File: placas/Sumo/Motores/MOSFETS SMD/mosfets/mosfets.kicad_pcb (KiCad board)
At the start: 2 copper layers, 37.3 x 39.4 mm, 18 parts, among them J1 Screw_Terminal_01x02, J3 Screw_Terminal_01x02, J5 Conn_01x06_Pin, Q1 IRLZ44N, Q2 IRLZ44N, Q3 IRLZ44N, Q4 IRLZ44N, U1 HIP4082xP

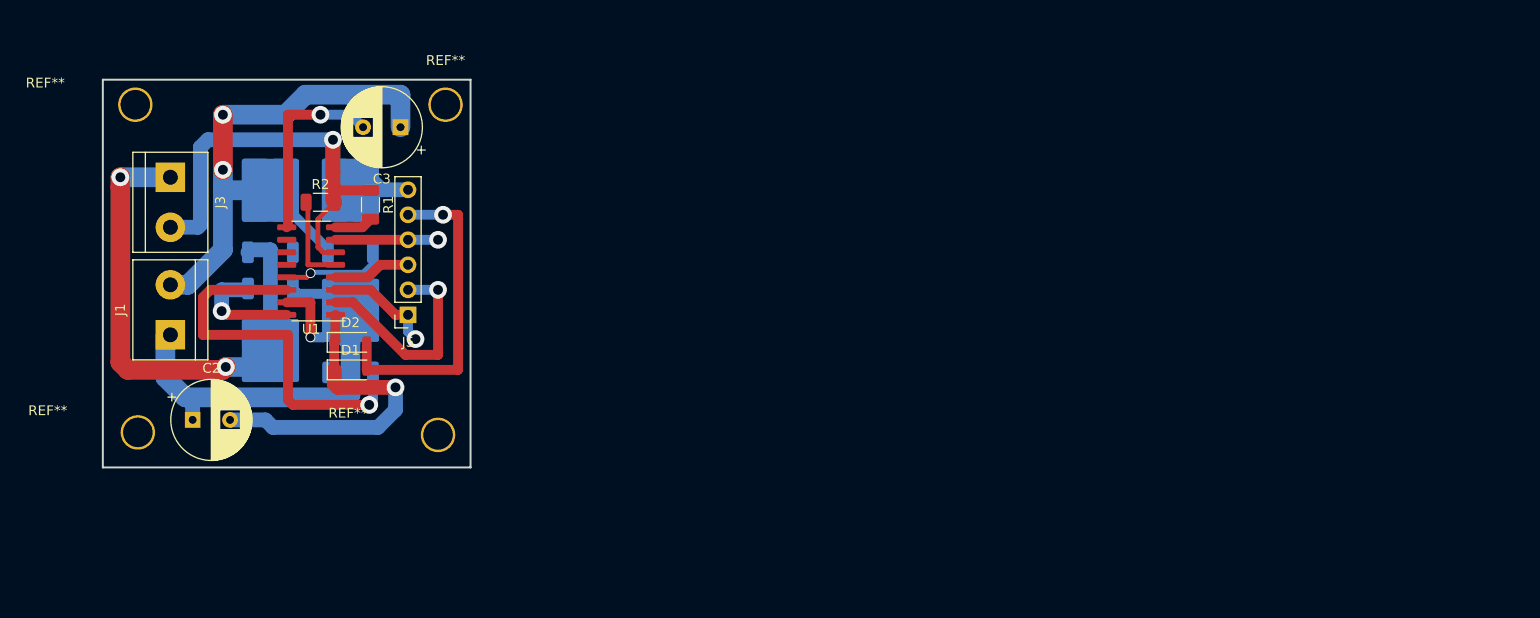
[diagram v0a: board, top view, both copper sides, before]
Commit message: dfg
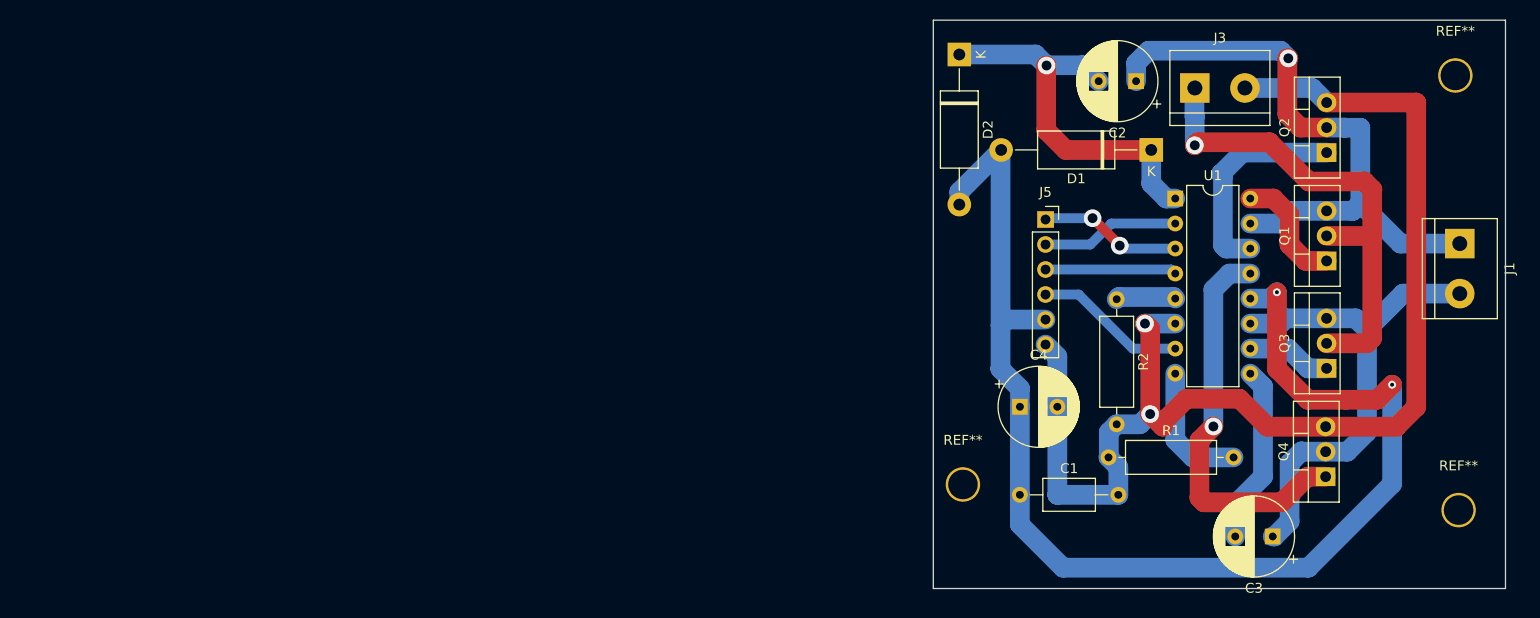
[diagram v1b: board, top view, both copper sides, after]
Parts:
- removed the REF** at (54.6, 52.8)
- removed the REF** at (24.1, 52.6)
- removed the REF** at (23.9, 19.3)
- removed the REF** at (55.4, 19.3)
- added C1: C, Capacitor_THT:C_Axial_L5.1mm_D3.1mm_P10.00mm_Horizontal, F.Cu at (113.7, 58.9)
- added C4: 47nf, Capacitor_THT:CP_Radial_D8.0mm_P3.80mm, F.Cu at (113.7, 50.0)
- added REF**: MountingHole_3.5mm_Pad, MountingHole:MountingHole_3.5mm_Pad, F.Cu at (158.2, 60.4)
- added REF**: MountingHole_3.5mm_Pad, MountingHole:MountingHole_3.5mm_Pad, F.Cu at (157.9, 16.3)
- added REF**: MountingHole_3.5mm_Pad, MountingHole:MountingHole_3.5mm_Pad, F.Cu at (107.9, 57.8)
- C2, C3: value C_Polarized -> 47nf
- D1, D2: footprint Diode_SMD:D_SOD-123 -> Diode_THT:D_DO-15_P15.24mm_Horizontal
- Q1, Q2, Q3, Q4: footprint Package_TO_SOT_SMD:TO-252-2 -> Package_TO_SOT_THT:TO-220-3_Vertical; moved to F.Cu
- R1, R2: value R -> 36k; footprint Resistor_SMD:R_1206_3216Metric -> Resistor_THT:R_Axial_DIN0309_L9.0mm_D3.2mm_P12.70mm_Horizontal
- U1: footprint Package_SO:SOIC-16_3.9x9.9mm_P1.27mm -> Package_DIP:DIP-16_W7.62mm
- moved J1 131.3 mm to (158.4, 33.4), turned to -90 degrees
- moved Q3 108.6 mm to (144.8, 46.0)
- moved Q1 107.5 mm to (144.8, 35.1), turned to 90 degrees
- moved J3 104.4 mm to (131.5, 17.6), turned to 0 degrees
- moved Q4 102.9 mm to (144.7, 57.0)
- moved C2 101.8 mm to (125.5, 16.9), turned to 180 degrees
- moved Q2 100.6 mm to (144.8, 24.1)
- moved C3 97.8 mm to (139.4, 63.1)
- moved U1 88.1 mm to (129.5, 28.8), turned to 0 degrees
- moved D1 84.3 mm to (127.0, 23.9), turned to 180 degrees
- moved R2 81.4 mm to (123.5, 39.0), turned to -90 degrees
- moved R1 79.2 mm to (122.7, 55.1), turned to 0 degrees
- moved D2 68.4 mm to (107.5, 14.2), turned to -90 degrees
- moved J5 65.5 mm to (116.3, 30.9), turned to 0 degrees
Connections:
- Q3 pad 2: Net-(J1-Pin_2) -> VDD
- Q3 pad 3: VDD -> Net-(J1-Pin_2)
- Q4 pad 2: GND -> Net-(J1-Pin_2)
- Q4 pad 3: Net-(J1-Pin_2) -> GND
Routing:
- net +5V: track 32.9 -> 128.6 mm, vias 1 -> 2
- net GND: track 53.7 -> 126.1 mm, vias 1 -> 2
- net Net-(Q4-G): track 10.4 -> 40.2 mm
- net Net-(Q2-G): track 39.8 -> 21.9 mm, vias 1 -> 0
- net Net-(U1-DIS): track 3.90 -> 13.4 mm
- net Net-(Q3-G): track 0.00 -> 8.58 mm
- net Net-(J5-Pin_2): track 22.3 -> 14.1 mm, vias 1 -> 0
- net Net-(D1-K): track 33.6 -> 39.9 mm
- net Net-(J1-Pin_1): track 69.0 -> 63.4 mm
- net Net-(J5-Pin_3): track 7.89 -> 13.3 mm
- net Net-(J5-Pin_4): track 10.4 -> 15.4 mm, vias 1 -> 0
- net Net-(J5-Pin_1): track 11.2 -> 14.5 mm, vias 1 -> 2
- net Net-(J1-Pin_2): track 54.4 -> 51.3 mm, vias 2 -> 0
- net Net-(U1-DEL): track 9.22 -> 6.11 mm
- net Net-(U1-AHB): track 19.6 -> 18.2 mm, vias 1 -> 0
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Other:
- board size 37.3 x 39.4 mm -> 58.1 x 57.7 mm
